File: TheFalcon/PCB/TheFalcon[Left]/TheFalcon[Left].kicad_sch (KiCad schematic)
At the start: 42 parts, among them J2 Conn_01x04_Pin, J3 Conn_01x04_Pin, J5 Conn_01x01, J6 Conn_01x01, SW1 SW_Push, SW2 SW_Push, U2 USBLC6-2P6, U3 USBLC6-2P6, U4 AMS1117-3.3, U6 STM32G431CBTx, Y1 X322516MOB4SI

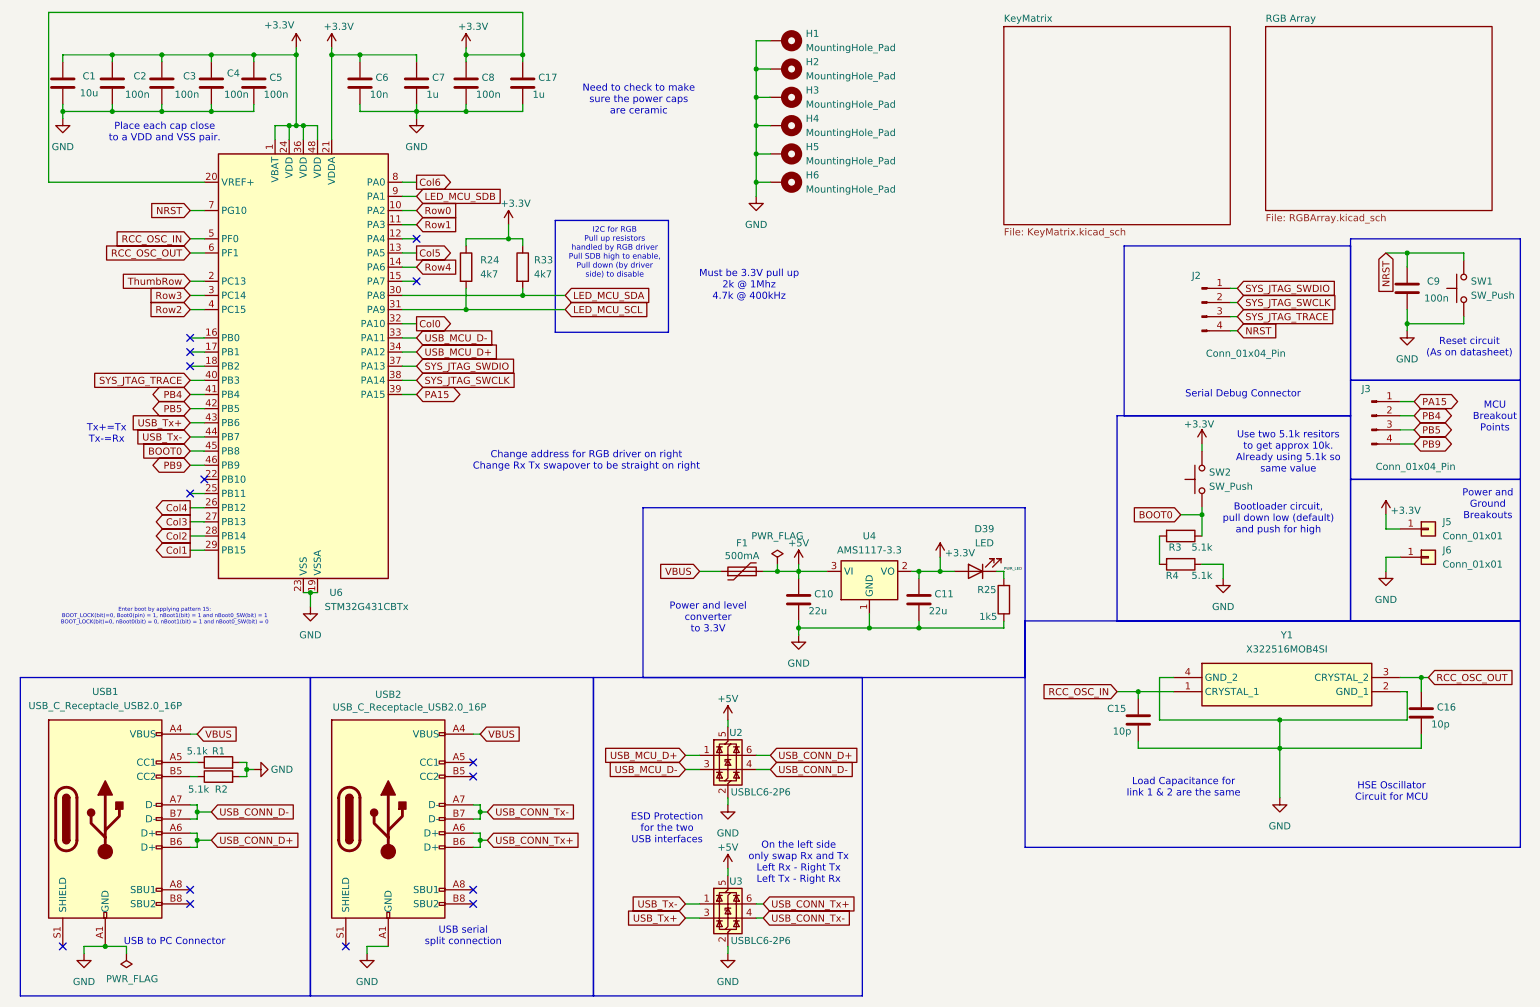
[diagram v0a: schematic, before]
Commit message: Cleaning up
I have all connections, just cleaning up
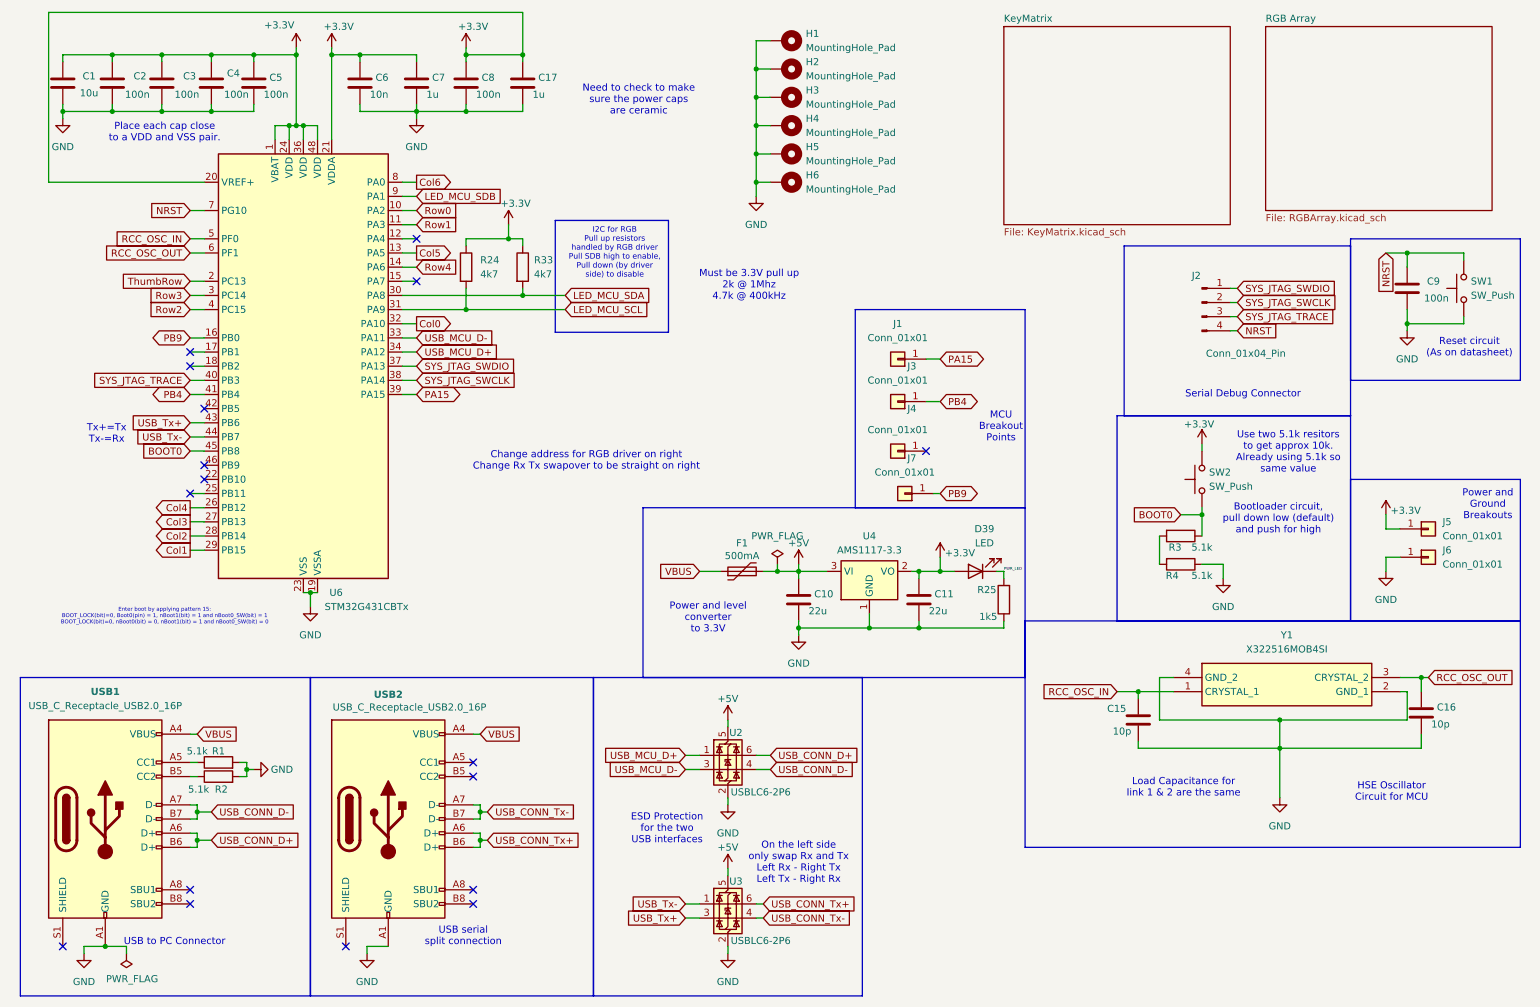
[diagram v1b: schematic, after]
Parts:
- removed J3: Conn_01x04_Pin, Connector_Wire:SolderWire-1sqmm_1x04_P5.4mm_D1.4mm_OD2.7mm, symbol Connector:Conn_01x04_Pin
- added J1, J3, J4, J7: Conn_01x01, Connector_Wire:SolderWire-0.1sqmm_1x01_D0.4mm_OD1mm, symbol Connector_Generic:Conn_01x01
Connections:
- net PA15: now also J1.1 (Pin_1)
- net PB4: now also J3.1 (Pin_1)
- net PB9: now also U6.16 (PB0), J7.1 (Pin_1); no longer U6.46 (PB9)
- net PB5: no longer names the net of U6.42 (PB5)
- no-connect marks 15 -> 17
